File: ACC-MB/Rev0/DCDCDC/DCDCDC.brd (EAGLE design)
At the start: 98.8 x 86.5 mm, 20 parts

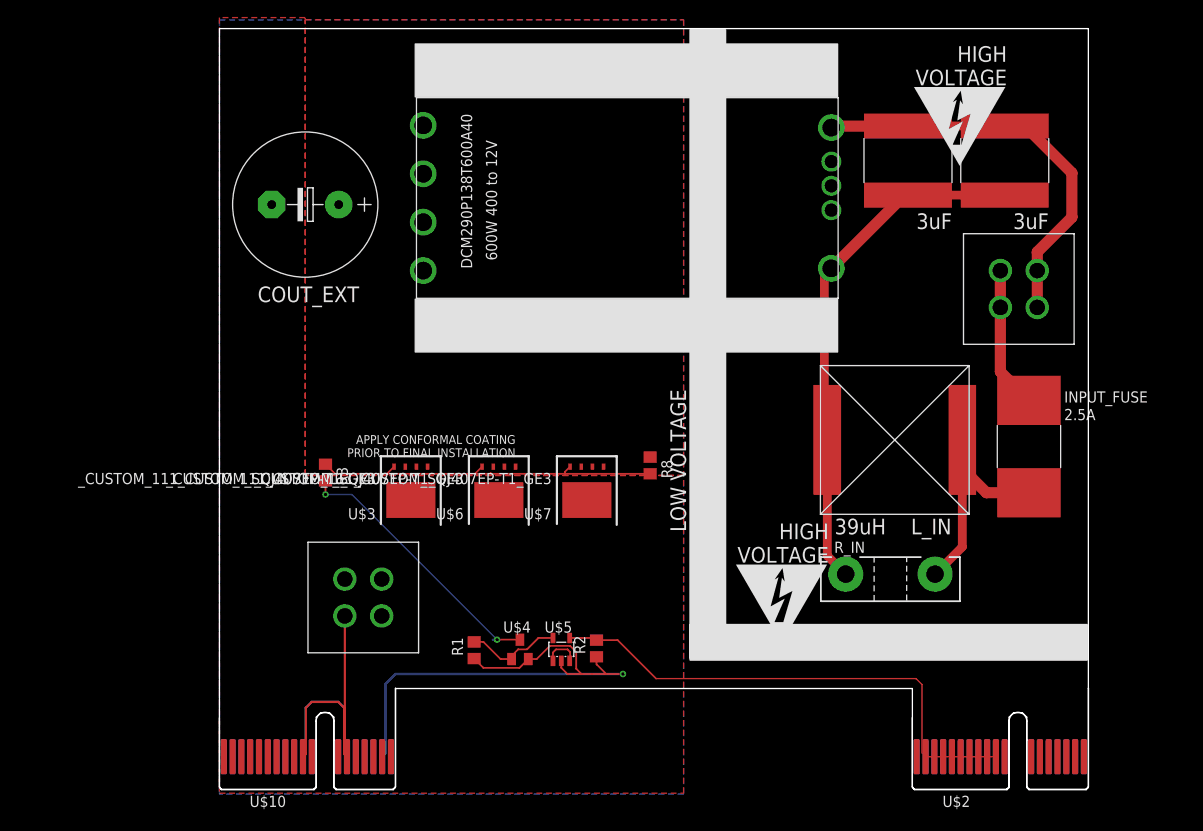
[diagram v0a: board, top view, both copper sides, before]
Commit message: brd
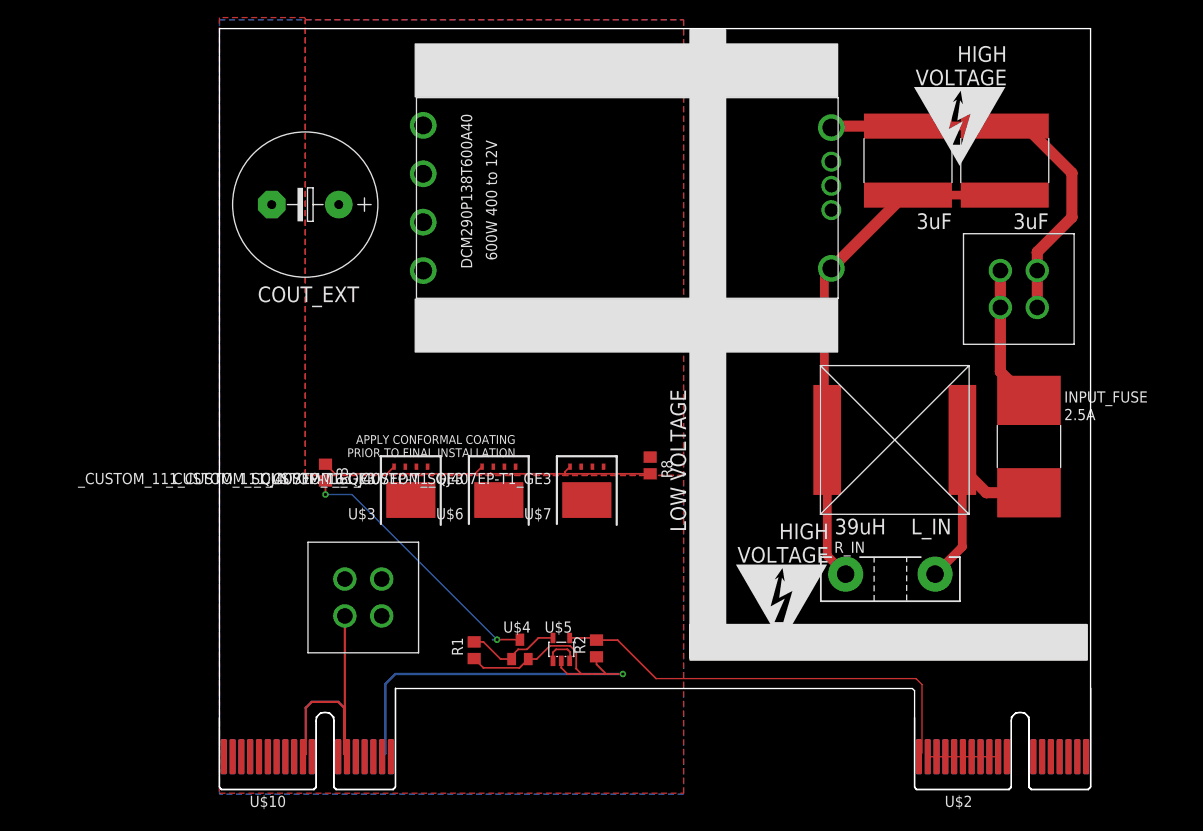
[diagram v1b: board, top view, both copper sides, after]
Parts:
- moved U$2 0.25 mm to (79.5, -11.5)
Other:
- board size 98.8 x 86.5 mm -> 99 x 86.5 mm
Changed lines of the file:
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@@
 <board>
 <plain>
-<wire x1="99" y1="75" x2="0.25" y2="75" width="0" layer="20"/>
-<wire x1="0.25" y1="75" x2="0.25" y2="0" width="0" layer="20"/>
+<wire x1="99.25" y1="75" x2="0.25" y2="75" width="0" layer="20"/>
+<wire x1="0.25" y1="75" x2="0.25" y2="-11.25" width="0" layer="20"/>
 <wire x1="20.25" y1="0" x2="79" y2="0" width="0" layer="20"/>
-<wire x1="99" y1="0" x2="99" y2="75" width="0" layer="20"/>
 <polygon width="0.1524" layer="21" pour="hatch">
 <vertex x="70.5" y="44.25"/>
@@
 <text x="33.9" y="28.8" size="1" layer="21" rot="R180">APPLY CONFORMAL COATING
 PRIOR TO FINAL INSTALLATION</text>
-<wire x1="0.25" y1="0" x2="0.25" y2="-11.25" width="0" layer="20"/>
 <wire x1="0.25" y1="-11.25" x2="0.5" y2="-11.5" width="0" layer="20"/>
 <wire x1="0.5" y1="-11.5" x2="11" y2="-11.5" width="0" layer="20"/>
@@
 <wire x1="20" y1="-11.5" x2="20.25" y2="-11.25" width="0" layer="20"/>
 <wire x1="20.25" y1="-11.25" x2="20.25" y2="0" width="0" layer="20"/>
-<wire x1="99" y1="0" x2="99" y2="-11.25" width="0" layer="20"/>
-<wire x1="99" y1="-11.25" x2="98.75" y2="-11.5" width="0" layer="20"/>
-<wire x1="98.75" y1="-11.5" x2="92.25" y2="-11.5" width="0" layer="20"/>
-<wire x1="92.25" y1="-11.5" x2="92" y2="-11.25" width="0" layer="20"/>
-<wire x1="92" y1="-11.25" x2="92" y2="-3.25" width="0" layer="20"/>
-<wire x1="92" y1="-3.25" x2="91.5" y2="-2.75" width="0" layer="20"/>
-<wire x1="91.5" y1="-2.75" x2="90.5" y2="-2.75" width="0" layer="20"/>
-<wire x1="90.5" y1="-2.75" x2="90" y2="-3.25" width="0" layer="20"/>
-<wire x1="90" y1="-3.25" x2="90" y2="-11.25" width="0" layer="20"/>
-<wire x1="90" y1="-11.25" x2="89.75" y2="-11.5" width="0" layer="20"/>
-<wire x1="89.75" y1="-11.5" x2="79.25" y2="-11.5" width="0" layer="20"/>
-<wire x1="79.25" y1="-11.5" x2="79" y2="-11.25" width="0" layer="20"/>
-<wire x1="79" y1="-11.25" x2="79" y2="0" width="0" layer="20"/>
 <polygon width="0.2" layer="21">
 <vertex x="57.75" y="3.5"/>
@@
 <vertex x="98.85" y="3.25"/>
 </polygon>
+<wire x1="99.25" y1="75" x2="99.25" y2="-11.25" width="0" layer="20"/>
+<wire x1="99.25" y1="-11.25" x2="99" y2="-11.5" width="0" layer="20"/>
+<wire x1="99" y1="-11.5" x2="92.5" y2="-11.5" width="0" layer="20"/>
+<wire x1="92.5" y1="-11.5" x2="92.25" y2="-11.25" width="0" layer="20"/>
+<wire x1="92.25" y1="-11.25" x2="92.25" y2="-3.25" width="0" layer="20"/>
+<wire x1="92.25" y1="-3.25" x2="91.75" y2="-2.75" width="0" layer="20"/>
+<wire x1="91.75" y1="-2.75" x2="90.75" y2="-2.75" width="0" layer="20"/>
+<wire x1="90.75" y1="-2.75" x2="90.25" y2="-3.25" width="0" layer="20"/>
+<wire x1="90.25" y1="-3.25" x2="90.25" y2="-11.25" width="0" layer="20"/>
+<wire x1="90.25" y1="-11.25" x2="90" y2="-11.5" width="0" layer="20"/>
+<wire x1="90" y1="-11.5" x2="79.5" y2="-11.5" width="0" layer="20"/>
+<wire x1="79.5" y1="-11.5" x2="79.25" y2="-11.25" width="0" layer="20"/>
+<wire x1="79.25" y1="-11.25" x2="79.25" y2="-0.25" width="0" layer="20"/>
+<wire x1="79.25" y1="-0.25" x2="79" y2="0" width="0" layer="20"/>
+<dimension x1="99.25" y1="75" x2="0.25" y2="75" x3="49.75" y3="80.5" textsize="1.778" layer="20"/>
 </plain>
 <attributes>
@@
 <element name="U$10" library="ACC-MB-R0" library_urn="urn:adsk.eagle:library:13324935" package="PCI-E_SLOT_36" value="PCIE-36-EDGE" x="0.5" y="-11.5"/>
 <element name="U$1" library="ACC-MB-R0" library_urn="urn:adsk.eagle:library:13324935" package="IPBT-102-H1-T-D" package3d_urn="urn:adsk.eagle:package:13324986/2" value="IPBT-102-H1-T-D" x="14.5" y="8.25"/>
-<element name="U$2" library="ACC-MB-R0" library_urn="urn:adsk.eagle:library:13324935" package="PCI-E_SLOT_36" value="PCIE-36-EDGE" x="79.25" y="-11.5"/>
+<element name="U$2" library="ACC-MB-R0" library_urn="urn:adsk.eagle:library:13324935" package="PCI-E_SLOT_36" value="PCIE-36-EDGE" x="79.5" y="-11.5"/>
 </elements>
 <signals>
@@
 <contactref element="U$2" pad="B9"/>
 <contactref element="U$2" pad="B10"/>
-<wire x1="80.495" y1="-7.75" x2="88.495" y2="-7.75" width="0.1524" layer="1"/>
-<wire x1="87.495" y1="-7.75" x2="86.495" y2="-7.75" width="0" layer="19" extent="1-1"/>
-<wire x1="85.495" y1="-7.75" x2="86.495" y2="-7.75" width="0" layer="19" extent="1-1"/>
-<wire x1="84.495" y1="-7.75" x2="85.495" y2="-7.75" width="0" layer="19" extent="1-1"/>
-<wire x1="83.495" y1="-7.75" x2="84.495" y2="-7.75" width="0" layer="19" extent="1-1"/>
-<wire x1="82.495" y1="-7.75" x2="83.495" y2="-7.75" width="0" layer="19" extent="1-1"/>
-<wire x1="81.495" y1="-7.75" x2="82.495" y2="-7.75" width="0" layer="19" extent="1-1"/>
-<wire x1="88.495" y1="-7.75" x2="87.495" y2="-7.75" width="0" layer="19" extent="1-1"/>
-<wire x1="80.0922" y1="-7.3472" x2="80.495" y2="-7.75" width="0" layer="19" extent="1-1"/>
+<wire x1="80.745" y1="-7.75" x2="88.745" y2="-7.75" width="0.1524" layer="1"/>
+<wire x1="87.745" y1="-7.75" x2="86.745" y2="-7.75" width="0" layer="19" extent="1-1"/>
+<wire x1="85.745" y1="-7.75" x2="86.745" y2="-7.75" width="0" layer="19" extent="1-1"/>
+<wire x1="84.745" y1="-7.75" x2="85.745" y2="-7.75" width="0" layer="19" extent="1-1"/>
+<wire x1="83.745" y1="-7.75" x2="84.745" y2="-7.75" width="0" layer="19" extent="1-1"/>
+<wire x1="82.745" y1="-7.75" x2="83.745" y2="-7.75" width="0" layer="19" extent="1-1"/>
+<wire x1="81.745" y1="-7.75" x2="82.745" y2="-7.75" width="0" layer="19" extent="1-1"/>
+<wire x1="88.745" y1="-7.75" x2="87.745" y2="-7.75" width="0" layer="19" extent="1-1"/>
+<wire x1="80.0922" y1="-7.3472" x2="80.745" y2="-7.75" width="0" layer="19" extent="1-1"/>
 </signal>
 <signal name="N$3" class="1">

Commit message: update
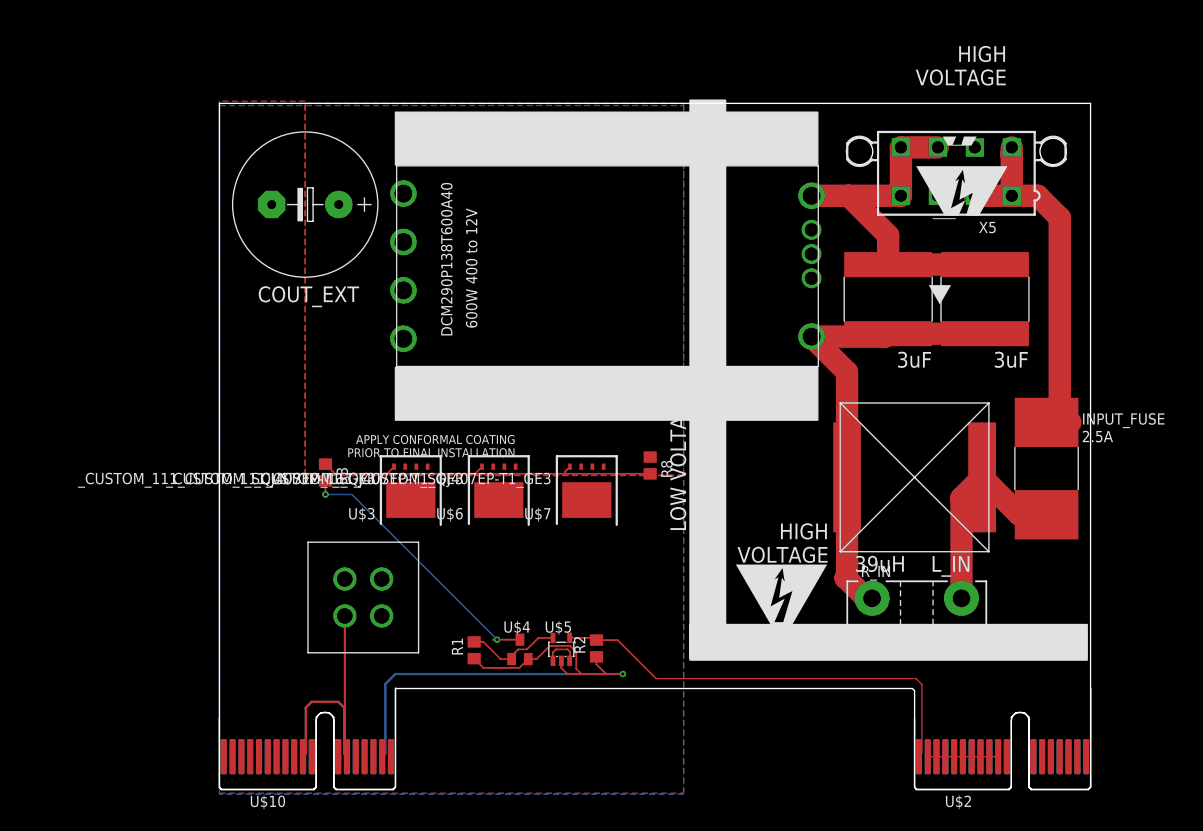
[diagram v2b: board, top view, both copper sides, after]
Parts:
- removed U$8: IPBT-102-H1-T-D, ACC-MB-R0:IPBT-102-H1-T-D
- added X5: 5566-8, con-molex:5566-8
- moved CFILTER_1 15.9 mm to (87.2, 44.2)
- moved CFILTER_2 15.9 mm to (76.2, 44.2)
- moved DCM290P138T600A40 8.07 mm to (44.4, 48.0)
- moved L_IN 4.81 mm to (79.2, 24.0)
- moved R_IN 4.07 mm to (79.5, 10.2)
- moved INPUT_FUSE 3.20 mm to (94.2, 25.0)
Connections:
- net V+: now also X5.1, X5.2, X5.5; no longer U$8.P$1, U$8.P$2
- net V-: now also X5.4, X5.7, X5.8; no longer U$8.P$3, U$8.P$4
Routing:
- net V+: track 16.1 -> 42.8 mm
- net V-: track 48.2 -> 42.2 mm
- net V+_FUSED: track 29.4 -> 28.1 mm
- net N$3: track 61.9 -> 62.6 mm
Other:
- board size 99 x 86.5 mm -> 99 x 78 mm
